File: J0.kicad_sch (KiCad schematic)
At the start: 0 parts

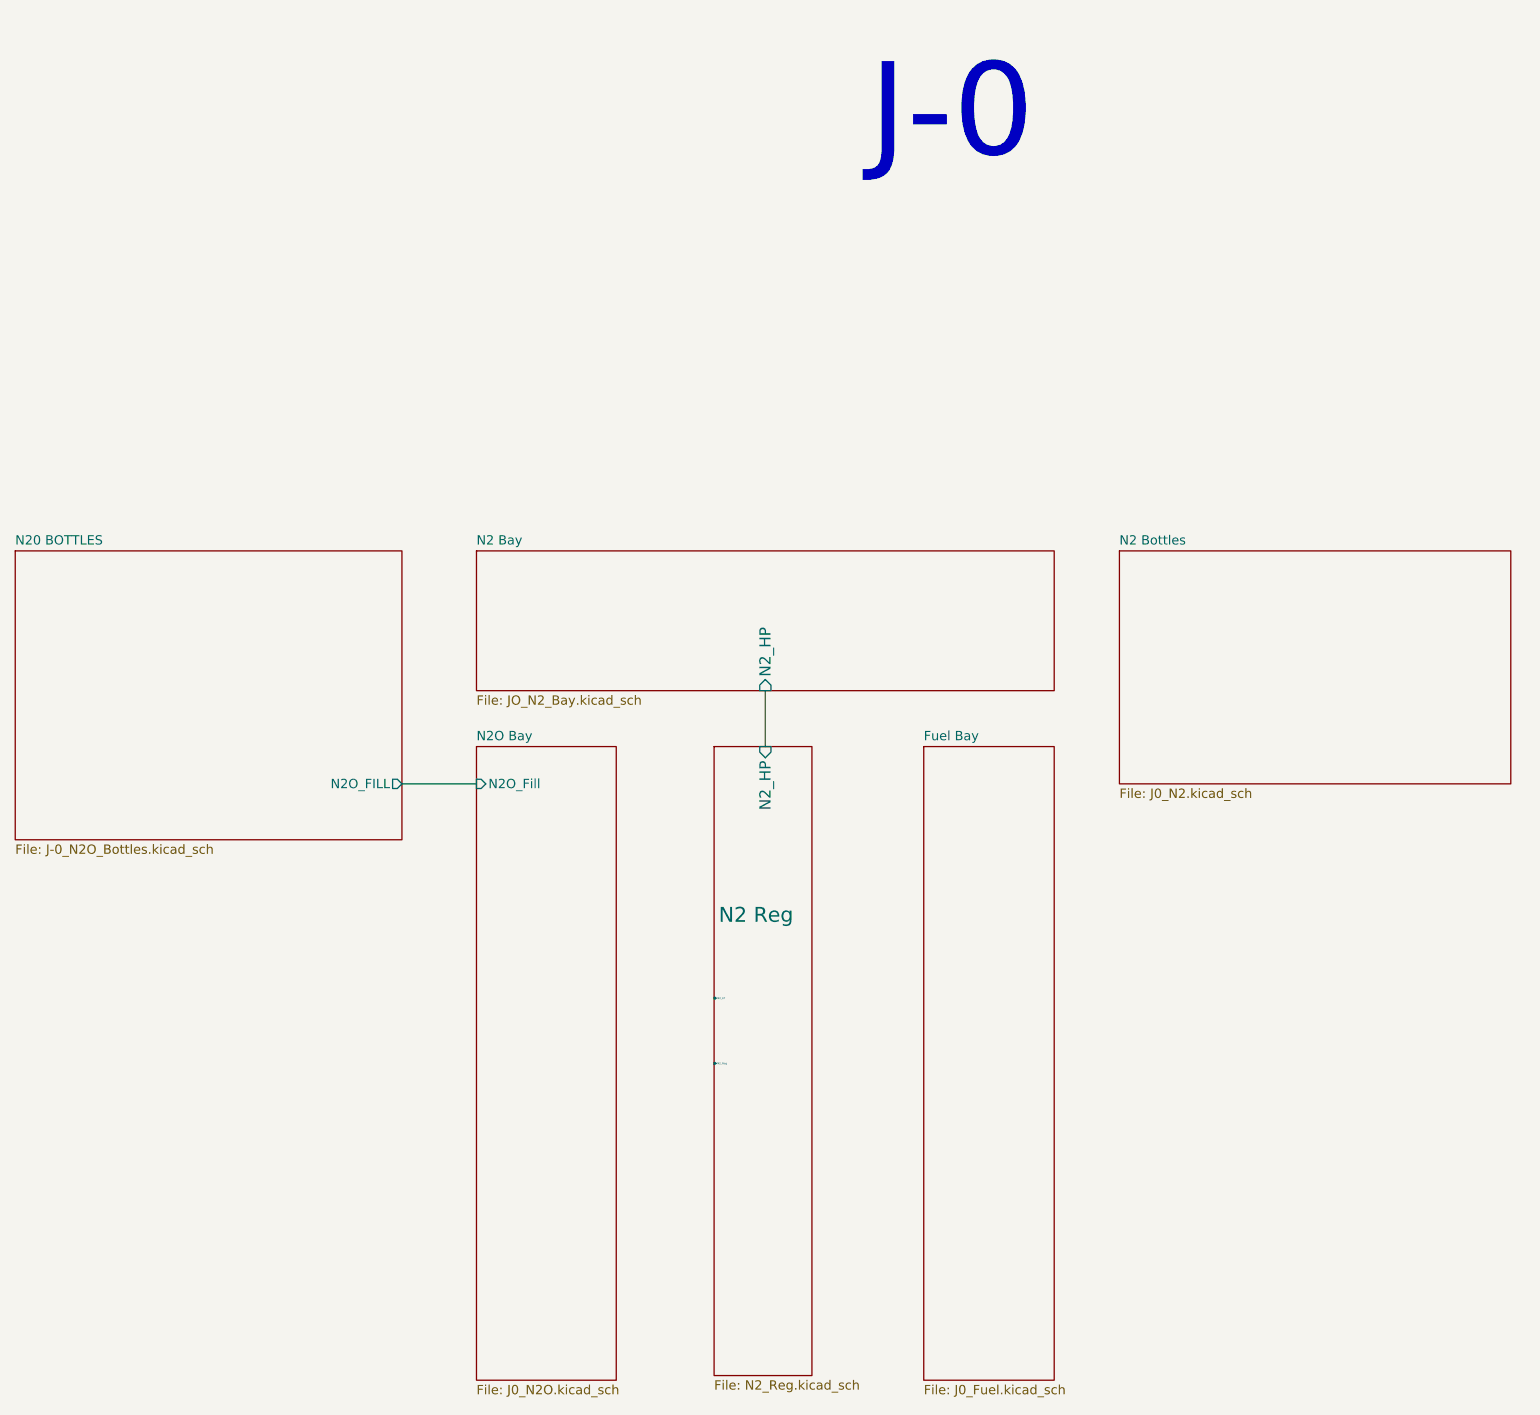
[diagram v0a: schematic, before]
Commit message: andrei it support
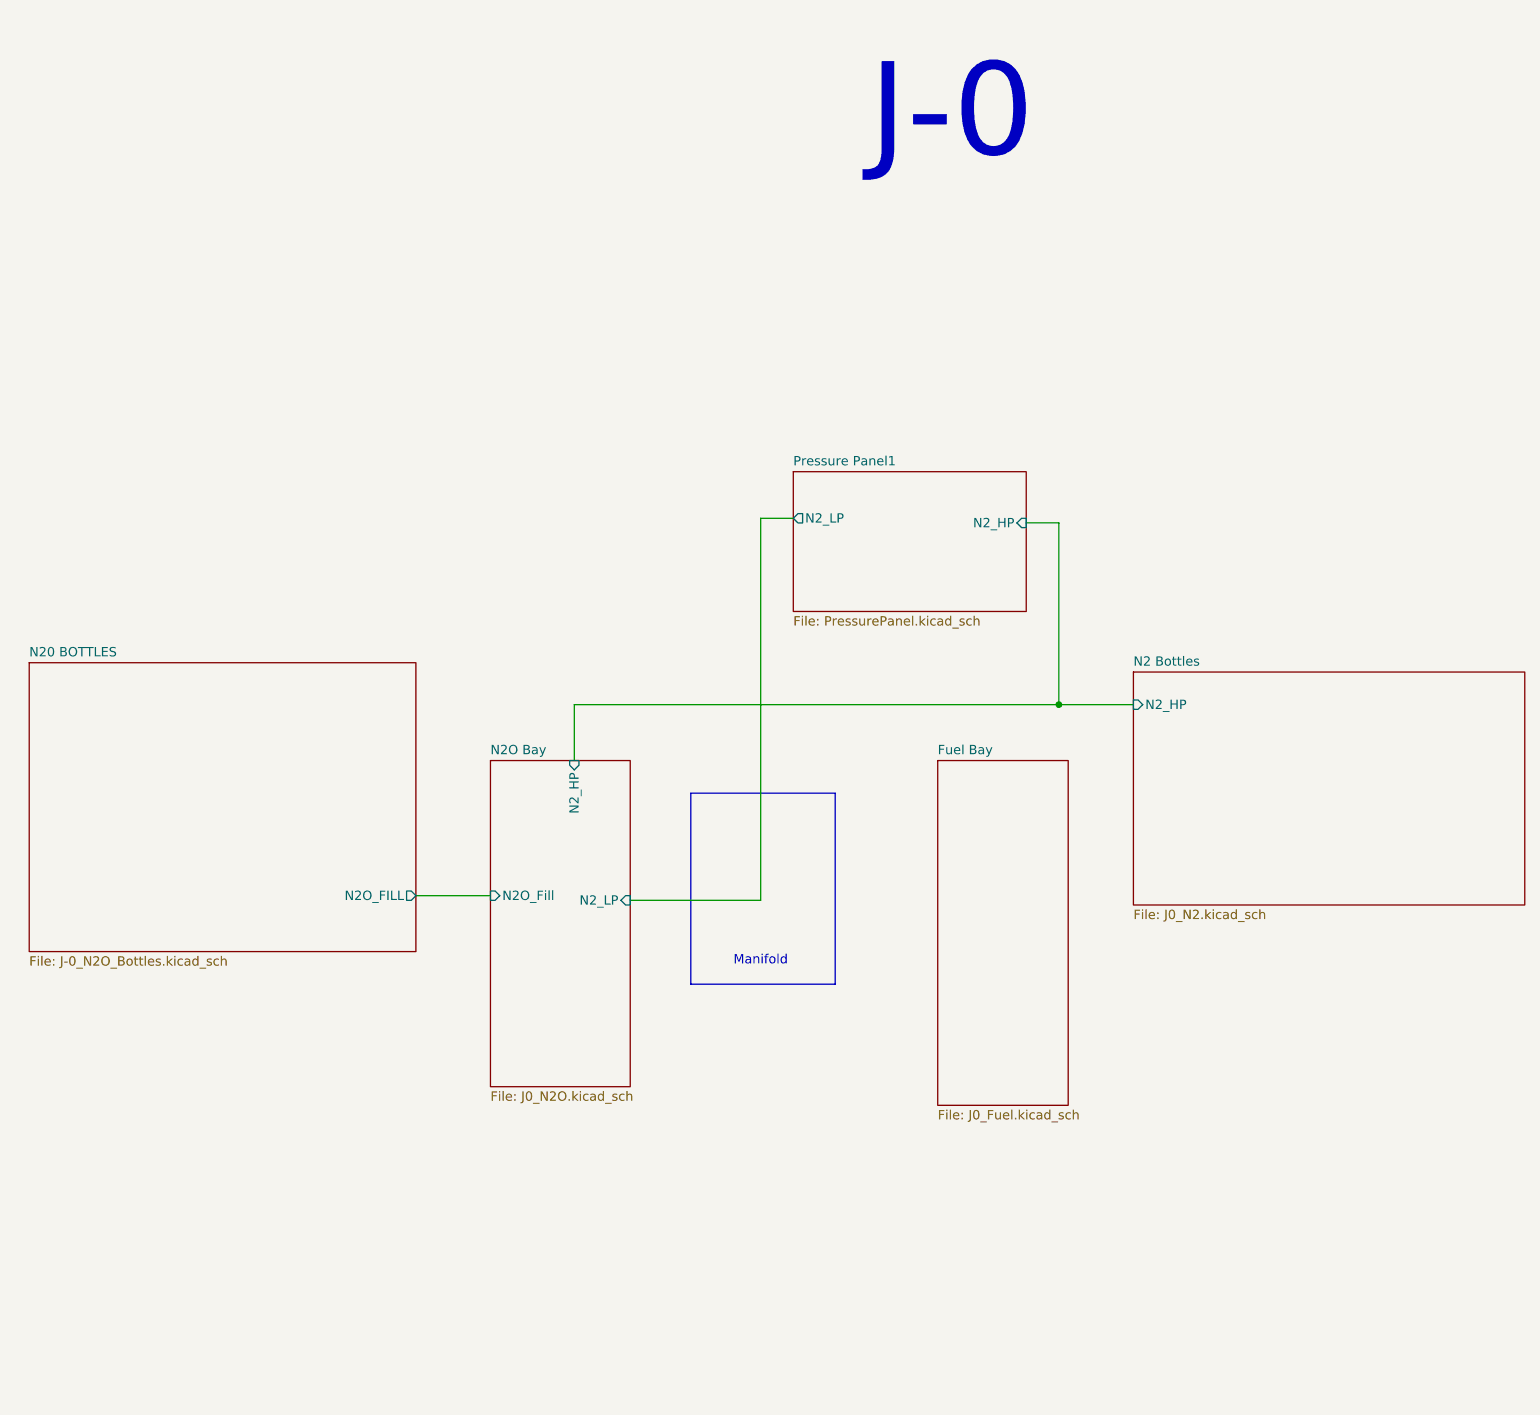
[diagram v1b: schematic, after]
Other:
- removed sheet N2 Bay
- removed sheet N2 Reg
- added sheet Pressure Panel1 (PressurePanel.kicad_sch)
- sheet N2 Bottles ports: added N2_HP; removed none
- sheet N2O Bay ports: added N2_HP, N2_LP; removed none
- note added: "Manifold"
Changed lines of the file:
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@@
 	(generator_version "9.0")
 	(paper "A4")
+	(rectangle
+		(start 123.19 81.28)
+		(end 142.875 107.315)
+		(stroke
+			(width 0)
+			(type default)
+		)
+		(fill
+			(type none)
+		)
+	)
+	(text "Manifold\n"
+		(exclude_from_sim no)
+		(at 132.715 104.14 0)
+		(effects
+			(font
+				(size 1.27 1.27)
+			)
+		)
+	)
 	(text "J-0\n"
 		(exclude_from_sim no)
@@
 		)
 	)
-	(wire
-		(pts
-			(xy 83.82 80.01) (xy 93.98 80.01)
+	(junction
+		(at 173.355 69.215)
+		(diameter 0)
+		(color 0 0 0 0)
+	)
+	(wire
+		(pts
+			(xy 132.715 43.815) (xy 132.715 95.885)
+		)
+		(stroke
+			(width 0)
+			(type default)
+		)
+	)
+	(wire
+		(pts
+			(xy 85.725 95.25) (xy 95.885 95.25)
 		)
 		(stroke
@@
 	(wire
 		(pts
-			(xy 133.35 67.31) (xy 133.35 74.93)
-		)
-		(stroke
-			(width 0)
-			(type default)
-		)
-	)
-	(sheet
-		(at 154.94 74.93)
-		(size 17.78 86.36)
+			(xy 168.91 44.45) (xy 173.355 44.45)
+		)
+		(stroke
+			(width 0)
+			(type default)
+		)
+	)
+	(wire
+		(pts
+			(xy 132.715 95.885) (xy 114.935 95.885)
+		)
+		(stroke
+			(width 0)
+			(type default)
+		)
+	)
+	(wire
+		(pts
+			(xy 137.16 43.815) (xy 132.715 43.815)
+		)
+		(stroke
+			(width 0)
+			(type default)
+		)
+	)
+	(wire
+		(pts
+			(xy 107.315 69.215) (xy 173.355 69.215)
+		)
+		(stroke
+			(width 0)
+			(type default)
+		)
+	)
+	(wire
+		(pts
+			(xy 173.355 44.45) (xy 173.355 69.215)
+		)
+		(stroke
+			(width 0)
+			(type default)
+		)
+	)
+	(wire
+		(pts
+			(xy 173.355 69.215) (xy 183.515 69.215)
+		)
+		(stroke
+			(width 0)
+			(type default)
+		)
+	)
+	(wire
+		(pts
+			(xy 107.315 69.215) (xy 107.315 76.835)
+		)
+		(stroke
+			(width 0)
+			(type default)
+		)
+	)
+	(sheet
+		(at 156.845 76.835)
+		(size 17.78 46.99)
 		(exclude_from_sim no)
 		(in_bom yes)
@@
 		)
 		(property "Sheetname" "Fuel Bay"
-			(at 154.94 74.2184 0)
+			(at 156.845 76.1234 0)
 			(effects
 				(font
@@
 		)
 		(property "Sheetfile" "J0_Fuel.kicad_sch"
-			(at 154.94 161.8746 0)
+			(at 156.845 124.4096 0)
 			(effects
 				(font
@@
 	)
 	(sheet
-		(at 93.98 74.93)
-		(size 19.05 86.36)
+		(at 95.885 76.835)
+		(size 19.05 44.45)
 		(exclude_from_sim no)
 		(in_bom yes)
@@
 		)
 		(property "Sheetname" "N2O Bay"
-			(at 93.98 74.2184 0)
+			(at 95.885 76.1234 0)
 			(effects
 				(font
@@
 		)
 		(property "Sheetfile" "J0_N2O.kicad_sch"
-			(at 93.98 161.8746 0)
+			(at 95.885 121.8696 0)
 			(effects
 				(font
@@
 		)
 		(pin "N2O_Fill" input
-			(at 93.98 80.01 180)
+			(at 95.885 95.25 180)
 			(effects
 				(font
@@
 			)
 		)
+		(pin "N2_HP" input
+			(at 107.315 76.835 90)
+			(effects
+				(font
+					(size 1.27 1.27)
+				)
+				(justify right)
+			)
+		)
+		(pin "N2_LP" input
+			(at 114.935 95.885 0)
+			(effects
+				(font
+					(size 1.27 1.27)
+				)
+				(justify right)
+			)
+		)
 		(instances
 			(project "P_IDs"
@@
 	)
 	(sheet
-		(at 93.98 48.26)
-		(size 78.74 19.05)
-		(exclude_from_sim no)
-		(in_bom yes)
-		(on_board yes)
-		(dnp no)
-		(fields_autoplaced yes)
-		(stroke
-			(width 0.1524)
-			(type solid)
-		)
-		(fill
-			(color 0 0 0 0.0000)
-		)
-		(property "Sheetname" "N2 Bay"
-			(at 93.98 47.5484 0)
-			(effects
-				(font
-					(size 1.27 1.27)
-				)
-				(justify left bottom)
-			)
-		)
-		(property "Sheetfile" "JO_N2_Bay.kicad_sch"
-			(at 93.98 67.8946 0)
+		(at 137.16 37.465)
+		(size 31.75 19.05)
+		(exclude_from_sim no)
+		(in_bom yes)
+		(on_board yes)
+		(dnp no)
+		(fields_autoplaced yes)
+		(stroke
+			(width 0.1524)
+			(type solid)
+		)
+		(fill
+			(color 0 0 0 0.0000)
+		)
+		(property "Sheetname" "Pressure Panel1"
+			(at 137.16 36.7534 0)
+			(effects
+				(font
+					(size 1.27 1.27)
+				)
+				(justify left bottom)
+			)
+		)
+		(property "Sheetfile" "PressurePanel.kicad_sch"
+			(at 137.16 57.0996 0)
 			(effects
 				(font
@@
 		)
 		(pin "N2_HP" input
-			(at 133.35 67.31 270)
-			(effects
-				(font
-					(size 1.524 1.524)
+			(at 168.91 44.45 0)
+			(effects
+				(font
+					(size 1.27 1.27)
+				)
+				(justify right)
+			)
+		)
+		(pin "N2_LP" output
+			(at 137.16 43.815 180)
+			(effects
+				(font
+					(size 1.27 1.27)
 				)
 				(justify left)
@@
 			(project "P_IDs"
 				(path "/045f1f05-3134-4b6d-91b6-463031104f1e/a0b6300e-76e9-4a18-afd6-e2d656b0d8f9/d375e00a-1ce3-4f93-9279-82acf09c7292"
-					(page "25")
-				)
-			)
-		)
-	)
-	(sheet
-		(at 31.115 48.26)
+					(page "2")
+				)
+			)
+		)
+	)
+	(sheet
+		(at 33.02 63.5)
 		(size 52.705 39.37)
 		(exclude_from_sim no)
@@
 		)
 		(property "Sheetname" "N20 BOTTLES"
-			(at 31.115 47.5484 0)
+			(at 33.02 62.7884 0)
 			(effects
 				(font
@@
 		)
 		(property "Sheetfile" "J-0_N2O_Bottles.kicad_sch"
-			(at 31.115 88.2146 0)
+			(at 33.02 103.4546 0)
 			(effects
 				(font
@@
 		)
 		(pin "N2O_FILL" output
-			(at 83.82 80.01 0)
+			(at 85.725 95.25 0)
 			(effects
 				(font
@@
 	)
 	(sheet
-		(at 181.61 48.26)
+		(at 183.515 64.77)
 		(size 53.34 31.75)
 		(exclude_from_sim no)
@@
 		)
 		(property "Sheetname" "N2 Bottles"
-			(at 181.61 47.5484 0)
+			(at 183.515 64.0584 0)
 			(effects
 				(font
@@
 		)
 		(property "Sheetfile" "J0_N2.kicad_sch"
-			(at 181.61 80.5946 0)
-			(effects
-				(font
-					(size 1.27 1.27)
-				)
-				(justify left top)
+			(at 183.515 97.1046 0)
+			(effects
+				(font
+					(size 1.27 1.27)
+				)
+				(justify left top)
+			)
+		)
+		(pin "N2_HP" input
+			(at 183.515 69.215 180)
+			(effects
+				(font
+					(size 1.27 1.27)
+				)
+				(justify left)
 			)
 		)
@@
 				)
 			)
-		)
-	)
-	(sheet
-		(at 126.365 74.93)
-		(size 13.335 85.725)
-		(exclude_from_sim no)
-		(in_bom yes)
-		(on_board yes)
-		(dnp no)
-		(stroke
-			(width 0.1524)
-			(type solid)
-		)
-		(fill
-			(color 0 0 0 0.0000)
-		)
-		(property "Sheetname" "N2 Reg"
-			(at 127 99.06 0)
-			(effects
-				(font
-					(size 2.032 2.032)
-				)
-				(justify left bottom)
-			)
-		)
-		(property "Sheetfile" "N2_Reg.kicad_sch"
-			(at 126.365 161.2396 0)
-			(effects
-				(font
-					(size 1.27 1.27)
-				)
-				(justify left top)
-			)
-		)
-		(pin "N2_HP" input
-			(at 133.35 74.93 90)
-			(effects
-				(font
-					(size 1.524 1.524)
-				)
-				(justify right)
-			)
-		)
-		(pin "N2_LP" input
-			(at 126.365 109.22 180)
-			(effects
-				(font
-					(size 0.254 0.254)
-				)
-				(justify left)
-			)
-		)
-		(pin "N2_Reg" input
-			(at 126.365 118.11 180)
-			(effects
-				(font
-					(size 0.254 0.254)
-				)
-				(justify left)
-			)
-		)
-		(instances
-			(project "P_IDs"
-				(path "/045f1f05-3134-4b6d-91b6-463031104f1e/a0b6300e-76e9-4a18-afd6-e2d656b0d8f9/d375e00a-1ce3-4f93-9279-82acf09c7292"
-					(page "26")
-				)
-			)
